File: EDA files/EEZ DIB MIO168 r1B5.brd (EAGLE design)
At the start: 146 x 95 mm, 302 parts, among them IC1 M24C32-WMN6P, IC10 DAC7760IPWPR, IC11 DAC7760IPWPR, IC12 OPA376AIDBVR, IC13 DAC7563TDGSR, IC14 OPA2196IDR, IC15 BTS3408G, IC16 BTS3408G, IC17 BTS3408G, IC18 BTS3408G, IC19 74HC126PW,118, IC2 Si8641BB-B-IS1, IC20 TL431B, IC21 DG468DV-T1-E3, IC22 DG468DV-T1-E3, IC23 DG468DV-T1-E3, IC24 DG468DV-T1-E3, IC25 DG468DV-T1-E3, IC26 DG468DV-T1-E3, IC27 DG468DV-T1-E3, IC28 DG468DV-T1-E3, IC29 DG468DV-T1-E3, IC3 Si8641BB-B-IS1, IC30 DG468DV-T1-E3, IC31 DG468DV-T1-E3, IC32 DG468DV-T1-E3, IC33 DG468DV-T1-E3, IC34 DG468DV-T1-E3, IC35 OPA376AIDBVR, IC36 ADS8674IDBT, IC4 L78L12, IC5 LM1117MP-5.0, IC6 LP2985-33DBVR, IC7 L79L12, IC8 STM32F446ZCT6, IC9 OPA2196IDR, J1 4907, J2 N.C., Q1 2N7002PS,115, Q10 BSS169, Q11 BSS169, Q12 BSS169, Q13 BSS169, Q2 2N7002PS,115, Q3 2N7002PS,115, Q4 2N7002PS,115, Q5 2N7002PS,115, Q6 BSS169, Q7 BSS169, Q8 BSS169, Q9 BSS169, X1 77317-104-28LF, X2 SSW-106-02-S-S, X3 691327310016, X4 691327310016, X5 1-2314878-0, X6 1-2314878-0, X7 1-2314878-0, Y1 25MHz

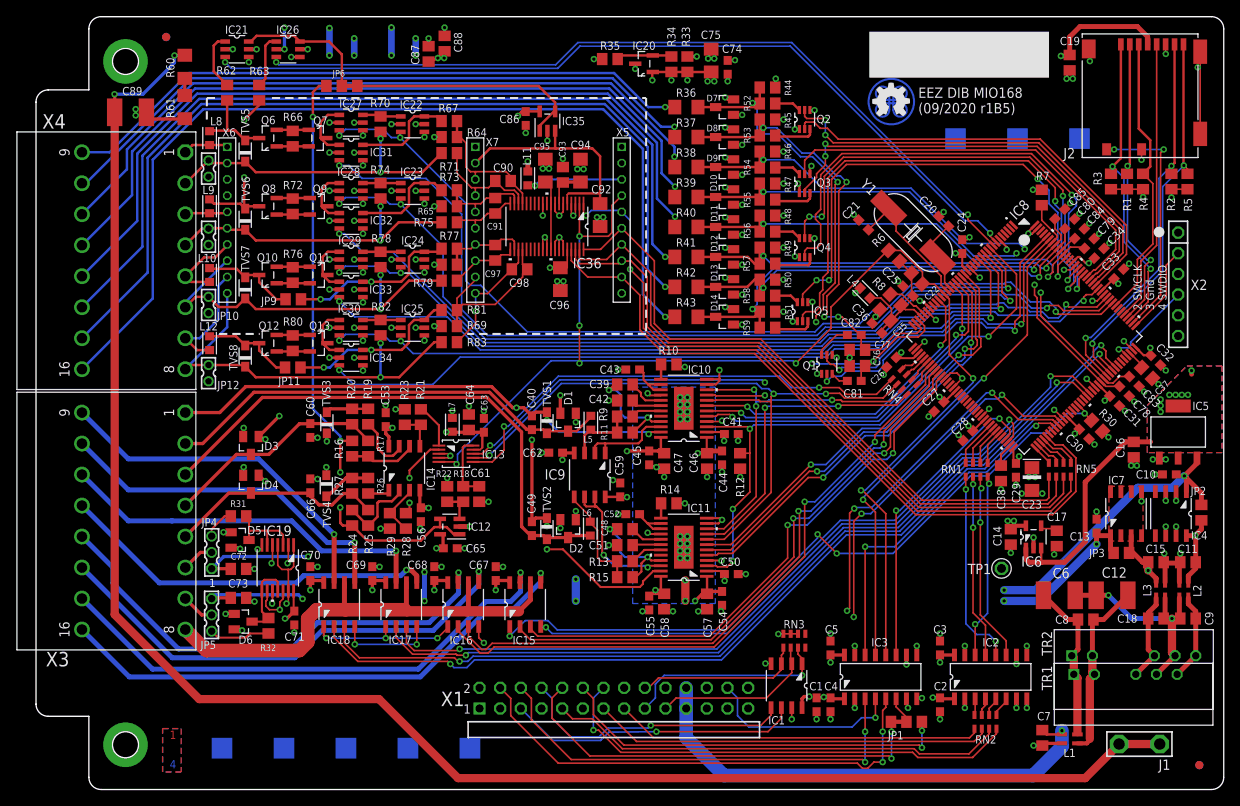
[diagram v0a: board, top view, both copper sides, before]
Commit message: #4, BOM update
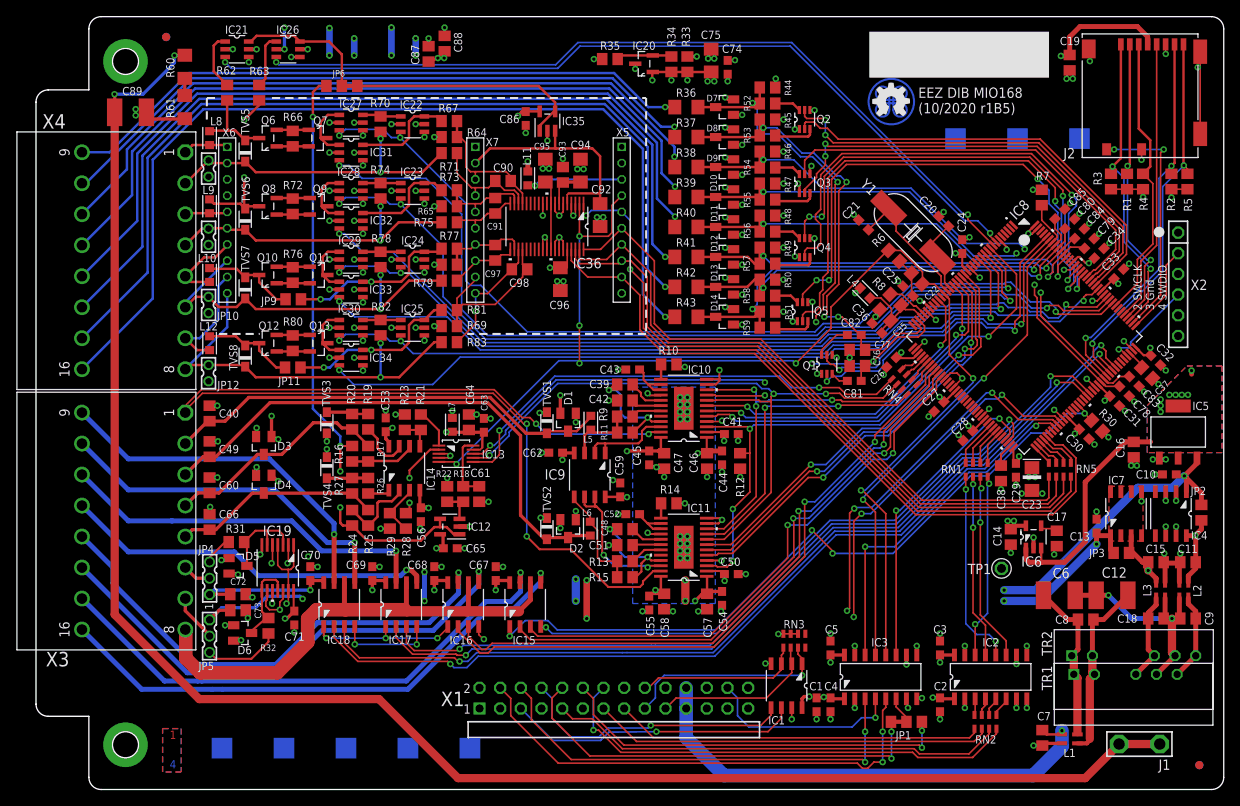
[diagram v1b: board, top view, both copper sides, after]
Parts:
- removed SH3: (no value), EEZ_Lib1:SHORT_NOHOLE
- C40, C49, C60, C66: value 100n -> 1n; device rcl:C0603 -> rcl:C0805
- moved C49 40.8 mm to (21.3, 41.8)
- moved SH2 40.7 mm to (18.4, 46.5), turned to 180 degrees
- moved C40 39.6 mm to (21.3, 46.2)
- moved C60 14.1 mm to (21.3, 37.4), turned to 90 degrees
- moved C66 13.2 mm to (21.3, 32.9)
- moved R31 3.19 mm to (24.6, 30.4)
- moved D5 3.19 mm to (24.8, 27.5)
- moved JP4 3.19 mm to (21.3, 26.0)
- moved C72 3.11 mm to (24.8, 24.0)
- moved JP5 2.62 mm to (21.3, 18.9)
- moved TVS4 2.22 mm to (35.8, 39.6)
- moved D3 1.59 mm to (28.0, 42.3)
- moved D4 1.59 mm to (28.0, 37.5)
- moved C73 1.53 mm to (24.8, 22.0)
- moved D6 1.40 mm to (25.4, 19.2)
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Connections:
- removed net -VSENSE1: C40.2, IC10.23, SH2.2, TVS1.C1
- removed net -VSENSE2: C49.2, IC11.23, SH3.2, TVS2.C1
- new net -VSENSE: IC10.23, IC11.23, SH2.2
- net GND: now also C40.2, C49.2, TVS1.C1, TVS2.C1; no longer SH3.1
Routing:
- net -VSENSE: track 0.00 -> 140.5 mm, vias 0 -> 4
- net GND: track 268.0 -> 228.3 mm, vias 178 -> 182
- net -VSENSE2: track 37.6 -> 0.00 mm, vias 4 -> 0
- net -VSENSE1: track 20.1 -> 0.00 mm, vias 2 -> 0
- net +3V3_ISO: track 98.6 -> 103.3 mm, vias 33 -> 35
- net N$1: track 69.2 -> 73.5 mm
- net -12V_ISO: track 258.7 -> 260.8 mm
- net N$40: track 7.53 -> 9.45 mm
- net +12V_ISO: track 264.3 -> 262.5 mm
- net N$39: track 4.07 -> 5.85 mm
- net DAC_OUT#2: track 67.9 -> 66.3 mm
- net POUT4: track 59.8 -> 61.4 mm
- net POUT5: track 60.1 -> 61.6 mm
- net N$73: track 27.0 -> 25.6 mm
- net POUT7: track 65.9 -> 67.2 mm
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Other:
- board text added: "EEZ DIB MIO168 (10/2020 r1B5)"
- board text added: "EEZ DIB MIO168 (10/2020 r1B5) Project source code: github.com/eez-open"
- board text removed: "EEZ DIB MIO168 (09/2020 r1B5)"
- board text removed: "EEZ DIB MIO168 (09/2020 r1B5) Project source code: github.com/eez-open"
